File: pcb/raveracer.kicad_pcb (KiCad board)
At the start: 2 copper layers, 125.1 x 44 mm, 15 parts, among them J1 System22_Video_PCB, J2 SCART-F, J3 DEBUG, J4 VGA-F, J5 Power Supply, U1 LM1881

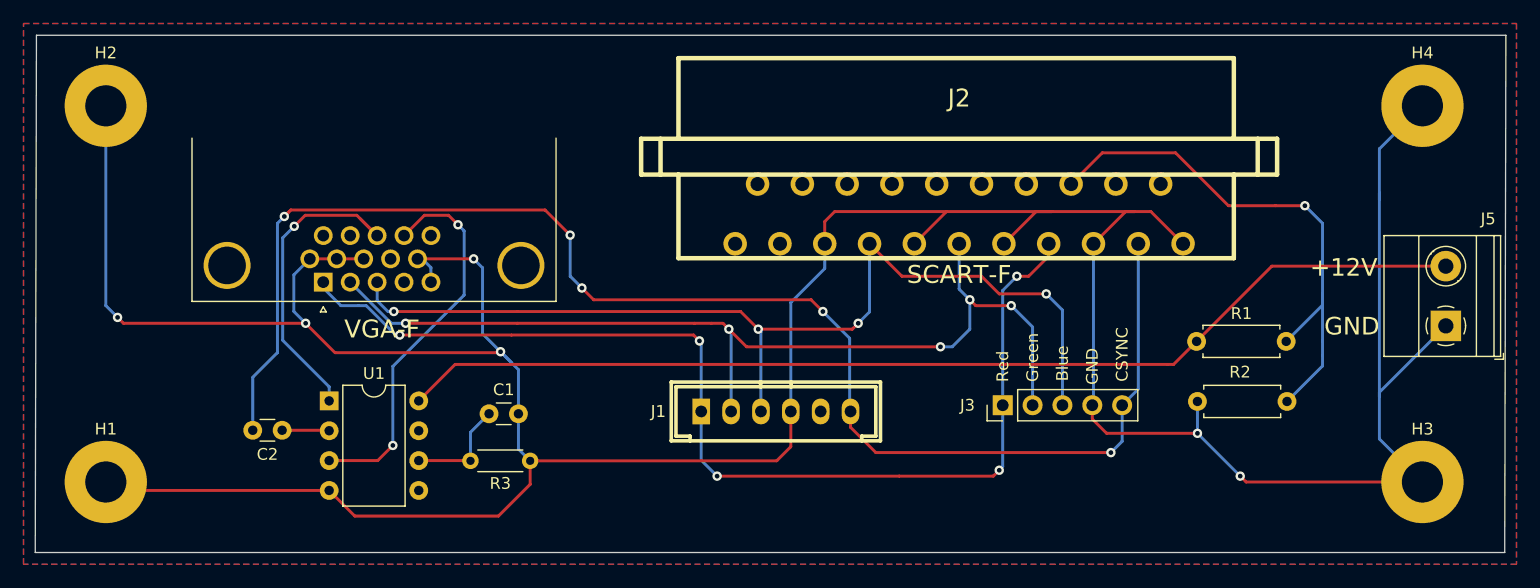
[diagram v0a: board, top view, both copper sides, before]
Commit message: finished routing of pcb
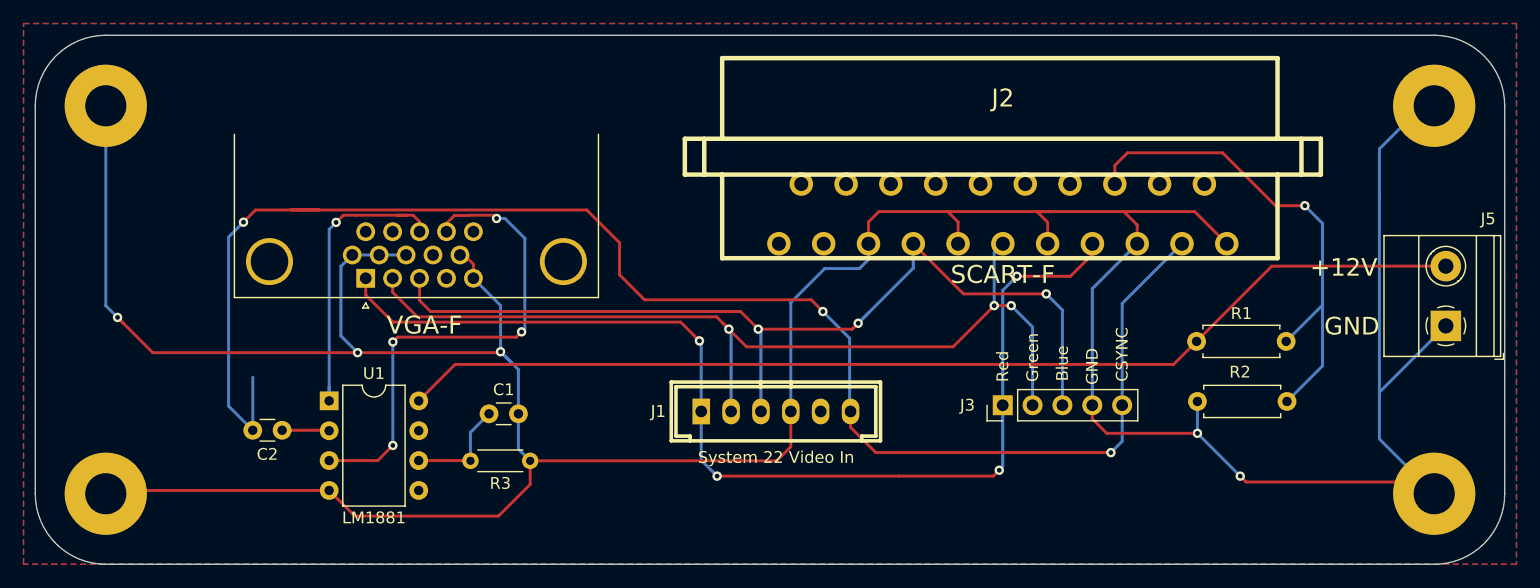
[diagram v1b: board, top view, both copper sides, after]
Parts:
- moved J2 3.72 mm to (82.3, 56.5)
- moved J4 3.63 mm to (28.1, 66.7)
- moved H3 1.41 mm to (119.0, 85.0)
- moved H1 1.00 mm to (6.00, 85.0)
- moved H4 1.00 mm to (119.0, 52.0)
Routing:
- net /CSYNC: track 124.6 -> 135.0 mm, vias 5 -> 3
- net Net-(J4-Pad14): track 33.1 -> 42.6 mm, vias 2 -> 4
- net /Blue: track 84.8 -> 80.7 mm, vias 4 -> 3
- net /Green: track 83.3 -> 79.8 mm, vias 5 -> 3
- net Net-(J2-Pad16): track 46.7 -> 43.9 mm
- net /Red: track 92.3 -> 93.7 mm, vias 5 -> 4
- net Net-(J4-Pad13): track 27.1 -> 25.8 mm
- net GND: track 313.0 -> 312.1 mm, vias 6 -> 5
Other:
- board size 125.1 x 44 mm -> 125 x 45 mm
- board text added: "System 22 Video In"
- board text added: "cascha coon 10/2020"
- board text removed: "cascha coon 09/2020"
